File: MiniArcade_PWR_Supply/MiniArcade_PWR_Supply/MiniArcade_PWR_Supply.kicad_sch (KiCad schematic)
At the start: 19 parts, among them IC1 MIC94310-SYM5-TR, J1 Conn_01x03, J2 Conn_01x02_Pin, J3 USB_C_PWR_Connector, U1 2479

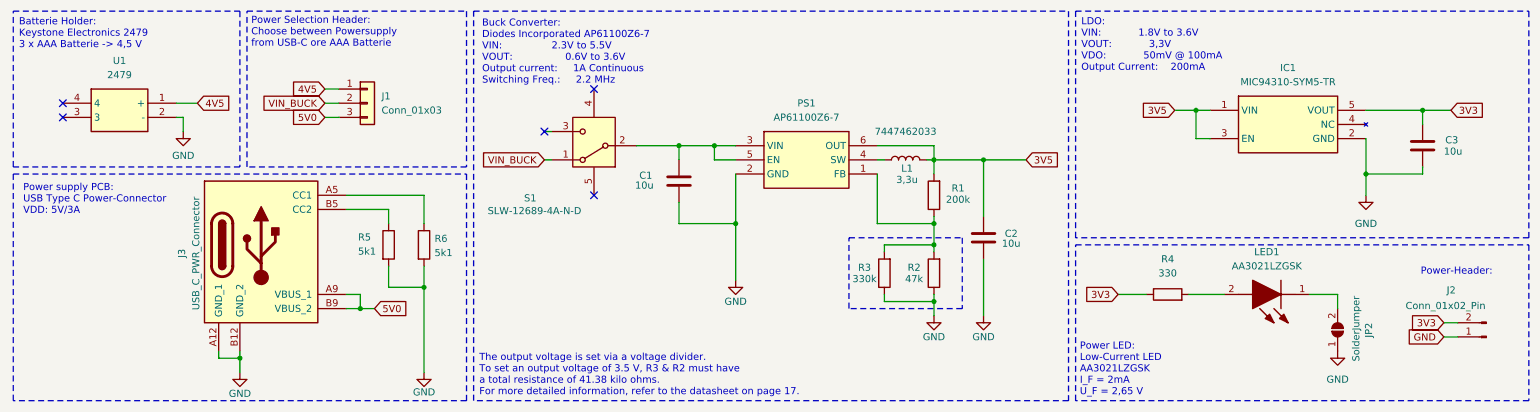
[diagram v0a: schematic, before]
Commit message: stand 03 11
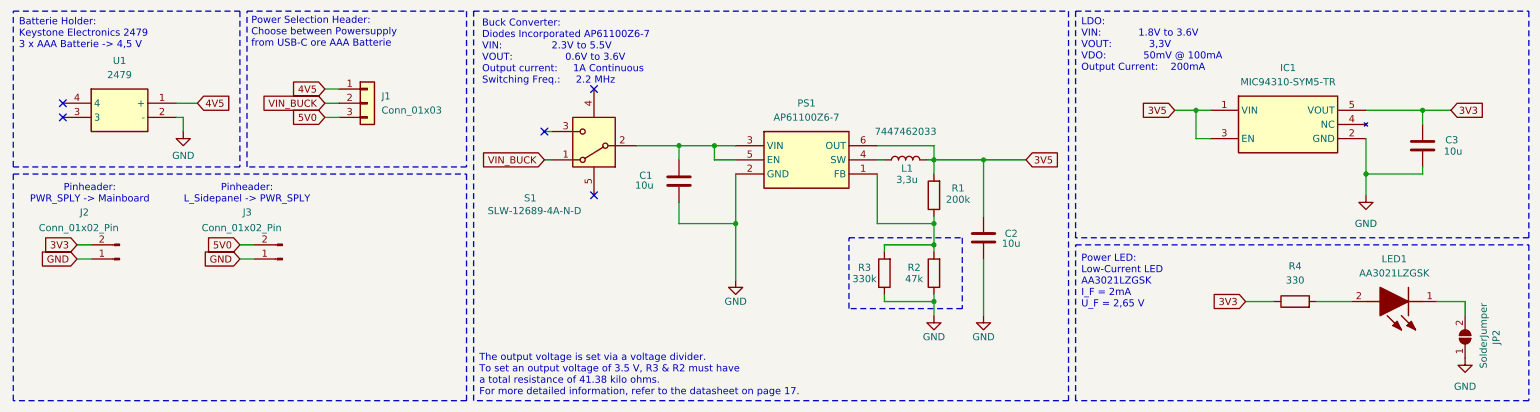
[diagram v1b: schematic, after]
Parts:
- removed J3: USB_C_PWR_Connector, MiniArcadePWRSupply:USB4125GFA, symbol MiniArcadePwrSupply:USB_C_PWR_CONNECTOR
- removed R5, R6: 5k1, Resistor_SMD:R_0603_1608Metric_Pad0.98x0.95mm_HandSolder, symbol Device:R
- added J3: Conn_01x02_Pin, Connector_PinHeader_1.00mm:PinHeader_1x02_P1.00mm_Horizontal, symbol Connector:Conn_01x02_Pin
- J1: footprint (none) -> Connector_PinHeader_1.00mm:PinHeader_1x03_P1.00mm_Vertical
- J2: footprint (none) -> Connector_PinHeader_1.00mm:PinHeader_1x02_P1.00mm_Horizontal
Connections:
- net 5V0: now also J3.2 (Pin_2)
- net GND: now also J3.1 (Pin_1)
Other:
- note added: "Pinheader: L_Sidepanel -> PWR_SPLY"
- note added: "Pinheader: PWR_SPLY -> Mainboard"
- note removed: "Power supply PCB: USB Type C Power-Connector VDD: 5V/3A"
- note removed: "Power-Header:"
- moved on the sheet: J2, JP2, LED1, R4

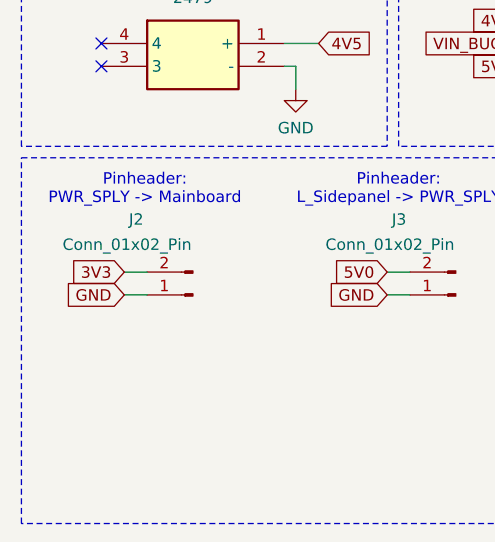
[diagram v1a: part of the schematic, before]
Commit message: 10 11 2025
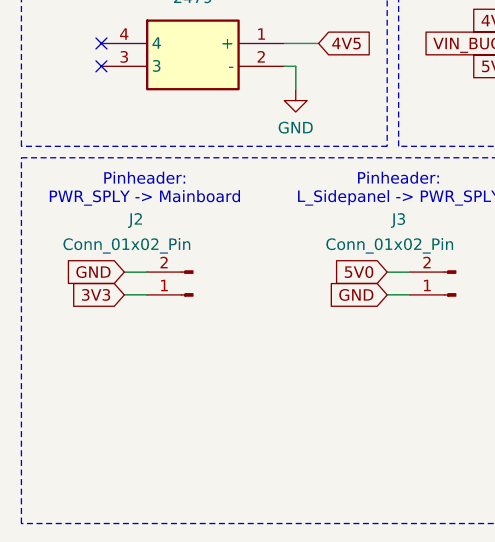
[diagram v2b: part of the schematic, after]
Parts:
- J2, J3: footprint Connector_PinHeader_1.00mm:PinHeader_1x02_P1.00mm_Horizontal -> Connector_PinHeader_2.54mm:PinHeader_1x02_P2.54mm_Horizontal
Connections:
- net 3V3: now also J2.1 (Pin_1); no longer J2.2 (Pin_2)
- net GND: now also J2.2 (Pin_2); no longer J2.1 (Pin_1)
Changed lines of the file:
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@@
+	(wire
+		(pts
+			(xy 132.08 39.37) (xy 132.08 36.83)
+		)
+		(stroke
+			(width 0)
+			(type default)
+		)
+	)
+	(wire
+		(pts
+			(xy 24.13 57.15) (xy 26.67 57.15)
+		)
+		(stroke
+			(width 0)
+			(type default)
+		)
+	)
+	(wire
+		(pts
+			(xy 138.43 39.37) (xy 138.43 36.83)
+		)
+		(stroke
+			(width 0)
+			(type default)
+		)
+	)
+	(wire
+		(pts
+			(xy 142.24 39.37) (xy 138.43 39.37)
+		)
+		(stroke
+			(width 0)
+			(type default)
+		)
+	)
 	(wire
 		(pts
 			(xy 24.13 54.61) (xy 26.67 54.61)
-		)
-		(stroke
-			(width 0)
-			(type default)
-		)
-	)
-	(wire
-		(pts
-			(xy 132.08 39.37) (xy 132.08 36.83)
-		)
-		(stroke
-			(width 0)
-			(type default)
-		)
-	)
-	(wire
-		(pts
-			(xy 24.13 57.15) (xy 26.67 57.15)
-		)
-		(stroke
-			(width 0)
-			(type default)
-		)
-	)
-	(wire
-		(pts
-			(xy 138.43 39.37) (xy 138.43 36.83)
-		)
-		(stroke
-			(width 0)
-			(type default)
-		)
-	)
-	(wire
-		(pts
-			(xy 142.24 39.37) (xy 138.43 39.37)
 		)
 		(stroke
@@
 		)
 	)
-	(global_label "GND"
-		(shape input)
-		(at 24.13 57.15 180)
-		(fields_autoplaced yes)
-		(effects
-			(font
-				(size 1.27 1.27)
-			)
-			(justify right)
-		)
-		(property "Intersheetrefs" "${INTERSHEET_REFS}"
-			(at 17.2743 57.15 0)
-			(effects
-				(font
-					(size 1.27 1.27)
-				)
-				(justify right)
-				(hide yes)
-			)
-		)
-	)
 	(global_label "3V5"
 		(shape input)
@@
 		)
 	)
+	(global_label "GND"
+		(shape input)
+		(at 24.13 54.61 180)
+		(fields_autoplaced yes)
+		(effects
+			(font
+				(size 1.27 1.27)
+			)
+			(justify right)
+		)
+		(property "Intersheetrefs" "${INTERSHEET_REFS}"
+			(at 17.2743 54.61 0)
+			(effects
+				(font
+					(size 1.27 1.27)
+				)
+				(justify right)
+				(hide yes)
+			)
+		)
+	)
 	(global_label "3V3"
 		(shape input)
@@
 	(global_label "3V3"
 		(shape input)
-		(at 24.13 54.61 180)
+		(at 24.13 57.15 180)
 		(fields_autoplaced yes)
 		(effects
@@
 		)
 		(property "Intersheetrefs" "${INTERSHEET_REFS}"
-			(at 17.6372 54.61 0)
+			(at 17.6372 57.15 0)
 			(effects
 				(font
@@
 			)
 		)
-		(property "Footprint" "Connector_PinHeader_1.00mm:PinHeader_1x02_P1.00mm_Horizontal"
+		(property "Footprint" "Connector_PinHeader_2.54mm:PinHeader_1x02_P2.54mm_Horizontal"
 			(at 31.75 57.15 0)
 			(effects
@@
 			)
 		)
-		(property "Footprint" "Connector_PinHeader_1.00mm:PinHeader_1x02_P1.00mm_Horizontal"
+		(property "Footprint" "Connector_PinHeader_2.54mm:PinHeader_1x02_P2.54mm_Horizontal"
 			(at 60.96 57.15 0)
 			(effects

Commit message: 11 11 2025
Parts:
- J2, J3: footprint Connector_PinHeader_2.54mm:PinHeader_1x02_P2.54mm_Horizontal -> Connector_PinHeader_2.54mm:PinHeader_1x02_P2.54mm_Vertical

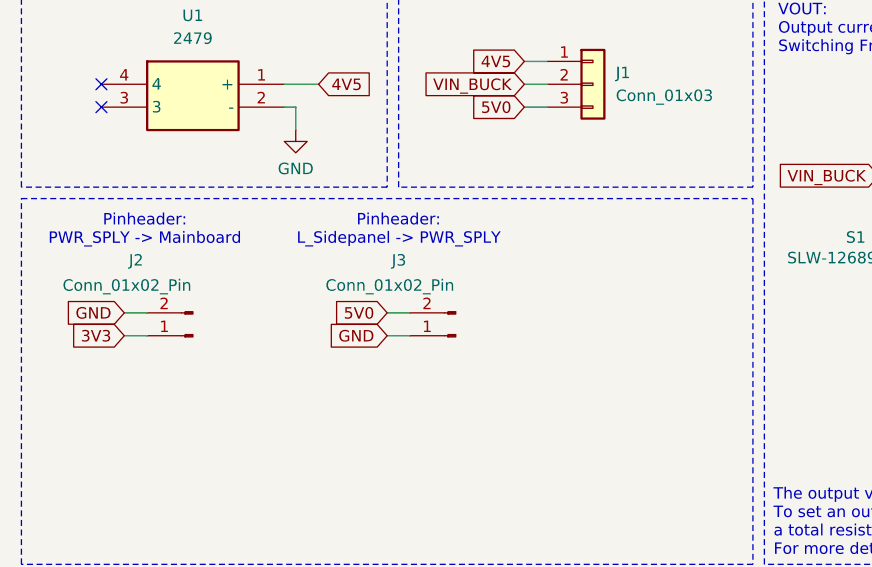
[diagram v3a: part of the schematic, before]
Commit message: 17 11 2025
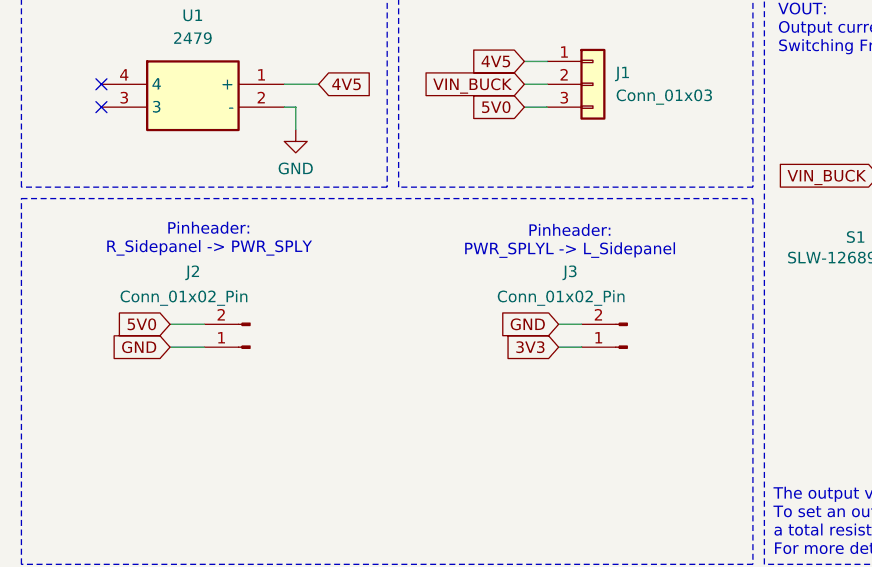
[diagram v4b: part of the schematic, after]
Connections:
- net 3V3: now also J3.1 (Pin_1); no longer J2.1 (Pin_1)
- net 5V0: now also J2.2 (Pin_2); no longer J3.2 (Pin_2)
- net GND: now also J2.1 (Pin_1), J3.2 (Pin_2); no longer J2.2 (Pin_2), J3.1 (Pin_1)
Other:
- note added: "Pinheader: PWR_SPLYL -> L_Sidepanel"
- note added: "Pinheader: R_Sidepanel -> PWR_SPLY"
- note removed: "Pinheader: L_Sidepanel -> PWR_SPLY"
- note removed: "Pinheader: PWR_SPLY -> Mainboard"
- moved on the sheet: J2, J3
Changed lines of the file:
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@@
 		)
 	)
-	(text "Pinheader:\nPWR_SPLY -> Mainboard\n"
+	(text "Pinheader:\nR_Sidepanel -> PWR_SPLY \n"
 		(exclude_from_sim no)
-		(at 26.416 45.466 0)
+		(at 33.528 46.482 0)
 		(effects
 			(font
@@
 		)
 	)
-	(text "Pinheader:\nL_Sidepanel -> PWR_SPLY\n\n"
+	(text "Pinheader:\nPWR_SPLYL -> L_Sidepanel\n\n"
 		(exclude_from_sim no)
-		(at 54.61 46.482 0)
+		(at 73.66 47.752 0)
 		(effects
 			(font
@@
 	(wire
 		(pts
-			(xy 68.58 31.75) (xy 71.12 31.75)
+			(xy 72.39 55.88) (xy 74.93 55.88)
 		)
 		(stroke
@@
 	(wire
 		(pts
-			(xy 68.58 29.21) (xy 71.12 29.21)
+			(xy 68.58 31.75) (xy 71.12 31.75)
 		)
 		(stroke
@@
 	(wire
 		(pts
-			(xy 68.58 26.67) (xy 71.12 26.67)
+			(xy 68.58 29.21) (xy 71.12 29.21)
 		)
 		(stroke
@@
 	(wire
 		(pts
-			(xy 265.43 41.91) (xy 255.27 41.91)
+			(xy 68.58 26.67) (xy 71.12 26.67)
 		)
 		(stroke
@@
 	(wire
 		(pts
-			(xy 53.34 54.61) (xy 55.88 54.61)
+			(xy 265.43 41.91) (xy 255.27 41.91)
 		)
 		(stroke
@@
 	(wire
 		(pts
-			(xy 24.13 57.15) (xy 26.67 57.15)
+			(xy 138.43 39.37) (xy 138.43 36.83)
 		)
 		(stroke
@@
 	(wire
 		(pts
-			(xy 138.43 39.37) (xy 138.43 36.83)
+			(xy 142.24 39.37) (xy 138.43 39.37)
 		)
 		(stroke
@@
 	(wire
 		(pts
-			(xy 142.24 39.37) (xy 138.43 39.37)
+			(xy 167.64 50.8) (xy 177.8 50.8)
 		)
 		(stroke
@@
 	(wire
 		(pts
-			(xy 24.13 54.61) (xy 26.67 54.61)
+			(xy 273.05 64.77) (xy 273.05 67.31)
 		)
 		(stroke
@@
 	(wire
 		(pts
-			(xy 167.64 50.8) (xy 177.8 50.8)
+			(xy 267.97 64.77) (xy 273.05 64.77)
 		)
 		(stroke
@@
 	(wire
 		(pts
-			(xy 273.05 64.77) (xy 273.05 67.31)
+			(xy 29.21 58.42) (xy 33.02 58.42)
 		)
 		(stroke
@@
 	(wire
 		(pts
-			(xy 267.97 64.77) (xy 273.05 64.77)
+			(xy 132.08 46.99) (xy 132.08 50.8)
 		)
 		(stroke
@@
 	(wire
 		(pts
-			(xy 132.08 46.99) (xy 132.08 50.8)
+			(xy 177.8 64.77) (xy 177.8 67.31)
 		)
 		(stroke
@@
 	(wire
 		(pts
-			(xy 177.8 64.77) (xy 177.8 67.31)
+			(xy 265.43 40.64) (xy 265.43 41.91)
 		)
 		(stroke
@@
 	(wire
 		(pts
-			(xy 265.43 40.64) (xy 265.43 41.91)
+			(xy 255.27 35.56) (xy 255.27 41.91)
 		)
 		(stroke
@@
 	(wire
 		(pts
-			(xy 255.27 35.56) (xy 255.27 41.91)
+			(xy 72.39 58.42) (xy 74.93 58.42)
 		)
 		(stroke
@@
 	(wire
 		(pts
+			(xy 29.21 55.88) (xy 33.02 55.88)
+		)
+		(stroke
+			(width 0)
+			(type default)
+		)
+	)
+	(wire
+		(pts
 			(xy 177.8 39.37) (xy 186.69 39.37)
 		)
@@
 	(wire
 		(pts
-			(xy 53.34 57.15) (xy 55.88 57.15)
-		)
-		(stroke
-			(width 0)
-			(type default)
-		)
-	)
-	(wire
-		(pts
 			(xy 177.8 50.8) (xy 177.8 54.61)
 		)
@@
 	(global_label "GND"
 		(shape input)
-		(at 53.34 57.15 180)
+		(at 29.21 58.42 180)
 		(fields_autoplaced yes)
 		(effects
@@
 		)
 		(property "Intersheetrefs" "${INTERSHEET_REFS}"
-			(at 46.4843 57.15 0)
+			(at 22.3543 58.42 0)
 			(effects
 				(font
@@
 	(global_label "5V0"
 		(shape input)
-		(at 53.34 54.61 180)
+		(at 29.21 55.88 180)
 		(fields_autoplaced yes)
 		(effects
@@
 		)
 		(property "Intersheetrefs" "${INTERSHEET_REFS}"
-			(at 46.8472 54.61 0)
+			(at 22.7172 55.88 0)
 			(effects
 				(font
@@
 	(global_label "GND"
 		(shape input)
-		(at 24.13 54.61 180)
+		(at 72.39 55.88 180)
 		(fields_autoplaced yes)
 		(effects
@@
 		)
 		(property "Intersheetrefs" "${INTERSHEET_REFS}"
-			(at 17.2743 54.61 0)
+			(at 65.5343 55.88 0)
 			(effects
 				(font
@@
 	(global_label "3V3"
 		(shape input)
-		(at 24.13 57.15 180)
+		(at 72.39 58.42 180)
 		(fields_autoplaced yes)
 		(effects
@@
 		)
 		(property "Intersheetrefs" "${INTERSHEET_REFS}"
-			(at 17.6372 57.15 0)
+			(at 65.8972 58.42 0)
 			(effects
 				(font
@@
 	(symbol
 		(lib_id "Connector:Conn_01x02_Pin")
-		(at 31.75 57.15 180)
+		(at 38.1 58.42 180)
 		(unit 1)
 		(exclude_from_sim no)
@@
 		(dnp no)
 		(property "Reference" "J2"
-			(at 24.638 48.768 0)
+			(at 30.988 50.038 0)
 			(effects
 				(font
@@
 		)
 		(property "Value" "Conn_01x02_Pin"
-			(at 17.272 51.562 0)
+			(at 23.622 52.832 0)
 			(effects
 				(font
@@
 		)
 		(property "Footprint" "Connector_PinHeader_2.54mm:PinHeader_1x02_P2.54mm_Vertical"
-			(at 31.75 57.15 0)
+			(at 38.1 58.42 0)
 			(effects
 				(font
@@
 		)
 		(property "Datasheet" "~"
-			(at 31.75 57.15 0)
+			(at 38.1 58.42 0)
 			(effects
 				(font
@@
 		)
 		(property "Description" "Generic connector, single row, 01x02, script generated"
-			(at 31.75 57.15 0)
+			(at 38.1 58.42 0)
 			(effects
 				(font
@@
 		)
 		(property "Availability" ""
-			(at 31.75 57.15 0)
+			(at 38.1 58.42 0)
 			(effects
 				(font
@@
 		)
 		(property "Check_prices" ""
-			(at 31.75 57.15 0)
+			(at 38.1 58.42 0)
 			(effects
 				(font
@@
 		)
 		(property "Description_1" ""
-			(at 31.75 57.15 0)
+			(at 38.1 58.42 0)
 			(effects
 				(font
@@
 		)
 		(property "MANUFACTURER" ""
-			(at 31.75 57.15 0)
+			(at 38.1 58.42 0)
 			(effects
 				(font
@@
 		)
 		(property "MAXIMUM_PACKAGE_HEIGHT" ""
-			(at 31.75 57.15 0)
+			(at 38.1 58.42 0)
 			(effects
 				(font
@@
 		)
 		(property "MF" ""
-			(at 31.75 57.15 0)
+			(at 38.1 58.42 0)
 			(effects
 				(font
@@
 		)
 		(property "MP" ""
-			(at 31.75 57.15 0)
+			(at 38.1 58.42 0)
 			(effects
 				(font
@@
 		)
 		(property "PARTREV" ""
-			(at 31.75 57.15 0)
+			(at 38.1 58.42 0)
 			(effects
 				(font
@@
 		)
 		(property "Package" ""
-			(at 31.75 57.15 0)
+			(at 38.1 58.42 0)
 			(effects
 				(font
@@
 		)
 		(property "Price" ""
-			(at 31.75 57.15 0)
+			(at 38.1 58.42 0)
 			(effects
 				(font
@@
 		)
 		(property "STANDARD" ""
-			(at 31.75 57.15 0)
+			(at 38.1 58.42 0)
 			(effects
 				(font
@@
 		)
 		(property "SnapEDA_Link" ""
-			(at 31.75 57.15 0)
+			(at 38.1 58.42 0)
 			(effects
 				(font
@@
 	(symbol
 		(lib_id "Connector:Conn_01x02_Pin")
-		(at 60.96 57.15 180)
+		(at 80.01 58.42 180)
 		(unit 1)
 		(exclude_from_sim no)
@@
 		(dnp no)
 		(property "Reference" "J3"
-			(at 53.848 48.768 0)
+			(at 72.898 50.038 0)
 			(effects
 				(font
@@
 		)
 		(property "Value" "Conn_01x02_Pin"
-			(at 46.482 51.562 0)
+			(at 65.532 52.832 0)
 			(effects
 				(font
@@
 		)
 		(property "Footprint" "Connector_PinHeader_2.54mm:PinHeader_1x02_P2.54mm_Vertical"
-			(at 60.96 57.15 0)
+			(at 80.01 58.42 0)
 			(effects
 				(font
@@
 		)
 		(property "Datasheet" "~"
-			(at 60.96 57.15 0)
+			(at 80.01 58.42 0)
 			(effects
 				(font
@@
 		)
 		(property "Description" "Generic connector, single row, 01x02, script generated"
-			(at 60.96 57.15 0)
+			(at 80.01 58.42 0)
 			(effects
 				(font
@@
 		)
 		(property "Availability" ""
-			(at 60.96 57.15 0)
+			(at 80.01 58.42 0)
 			(effects
 				(font
@@
 		)
 		(property "Check_prices" ""
-			(at 60.96 57.15 0)
+			(at 80.01 58.42 0)
 			(effects
 				(font
@@
 		)
 		(property "Description_1" ""
-			(at 60.96 57.15 0)
+			(at 80.01 58.42 0)
 			(effects
 				(font
@@
 		)
 		(property "MANUFACTURER" ""
-			(at 60.96 57.15 0)
+			(at 80.01 58.42 0)
 			(effects
 				(font
@@
 		)
 		(property "MAXIMUM_PACKAGE_HEIGHT" ""
-			(at 60.96 57.15 0)
+			(at 80.01 58.42 0)
 			(effects
 				(font
@@
 		)
 		(property "MF" ""
-			(at 60.96 57.15 0)
+			(at 80.01 58.42 0)
 			(effects
 				(font
@@
 		)
 		(property "MP" ""
-			(at 60.96 57.15 0)
+			(at 80.01 58.42 0)
 			(effects
 				(font
@@
 		)
 		(property "PARTREV" ""
-			(at 60.96 57.15 0)
+			(at 80.01 58.42 0)
 			(effects
 				(font
@@
 		)
 		(property "Package" ""
-			(at 60.96 57.15 0)
+			(at 80.01 58.42 0)
 			(effects
 				(font
@@
 		)
 		(property "Price" ""
-			(at 60.96 57.15 0)
+			(at 80.01 58.42 0)
 			(effects
 				(font
@@
 		)
 		(property "STANDARD" ""
-			(at 60.96 57.15 0)
+			(at 80.01 58.42 0)
 			(effects
 				(font
@@
 		)
 		(property "SnapEDA_Link" ""
-			(at 60.96 57.15 0)
+			(at 80.01 58.42 0)
 			(effects
 				(font
